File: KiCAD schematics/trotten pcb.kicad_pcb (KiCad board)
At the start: 2 copper layers, 151 x 114.3 mm, 19 parts, among them J1 Conn_HRCU4_main, J2 Conn_screen_BRD_main, J3 Conn_screen_BRD_Slave, J4 Conn_01x04_Socket, J5 Conn_02x03_Odd_Even, SW1 Haut, SW2 Bas, SW3 MEM_1, SW4 MEM_2, U1 std:8a282036eb974780bd16e9b19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, U2 BOB-12009, U3 ADAFRUIT-ESP32-S3, U7 INA260

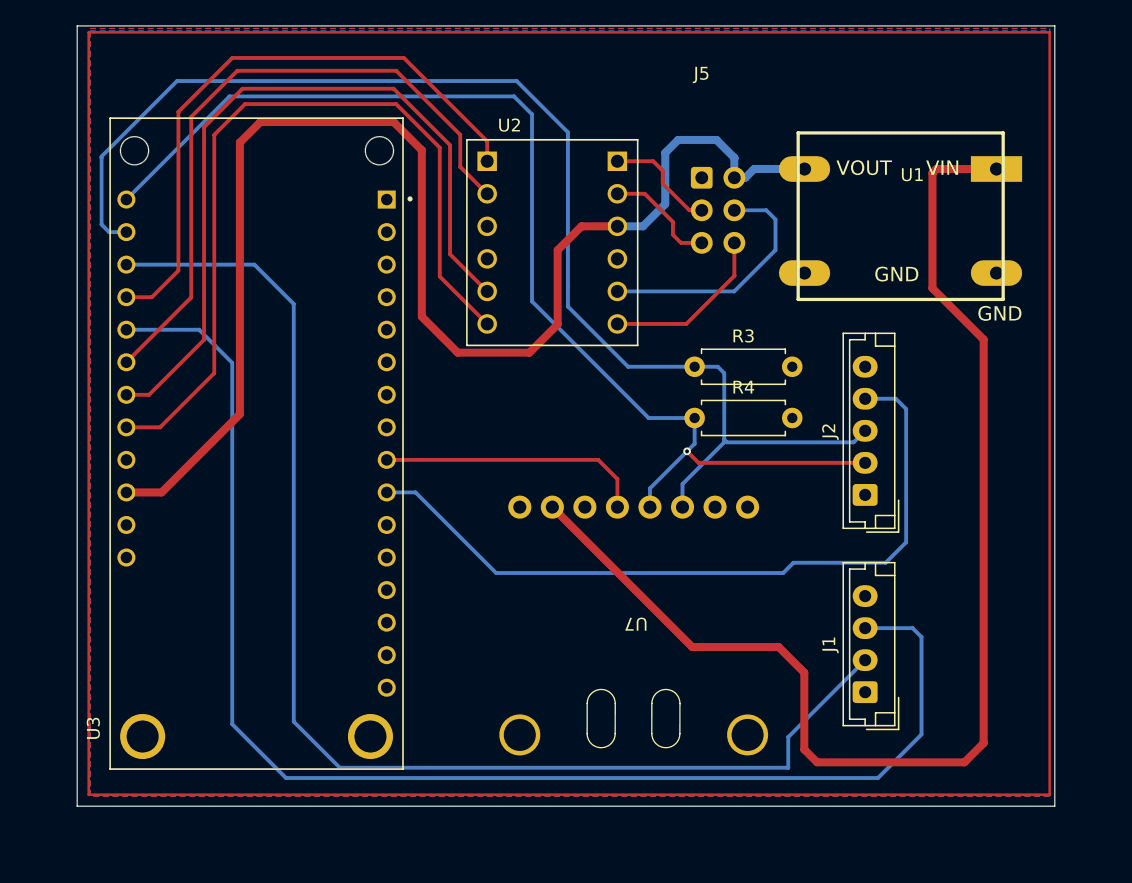
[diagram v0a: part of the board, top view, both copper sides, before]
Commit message: commencé le moteur
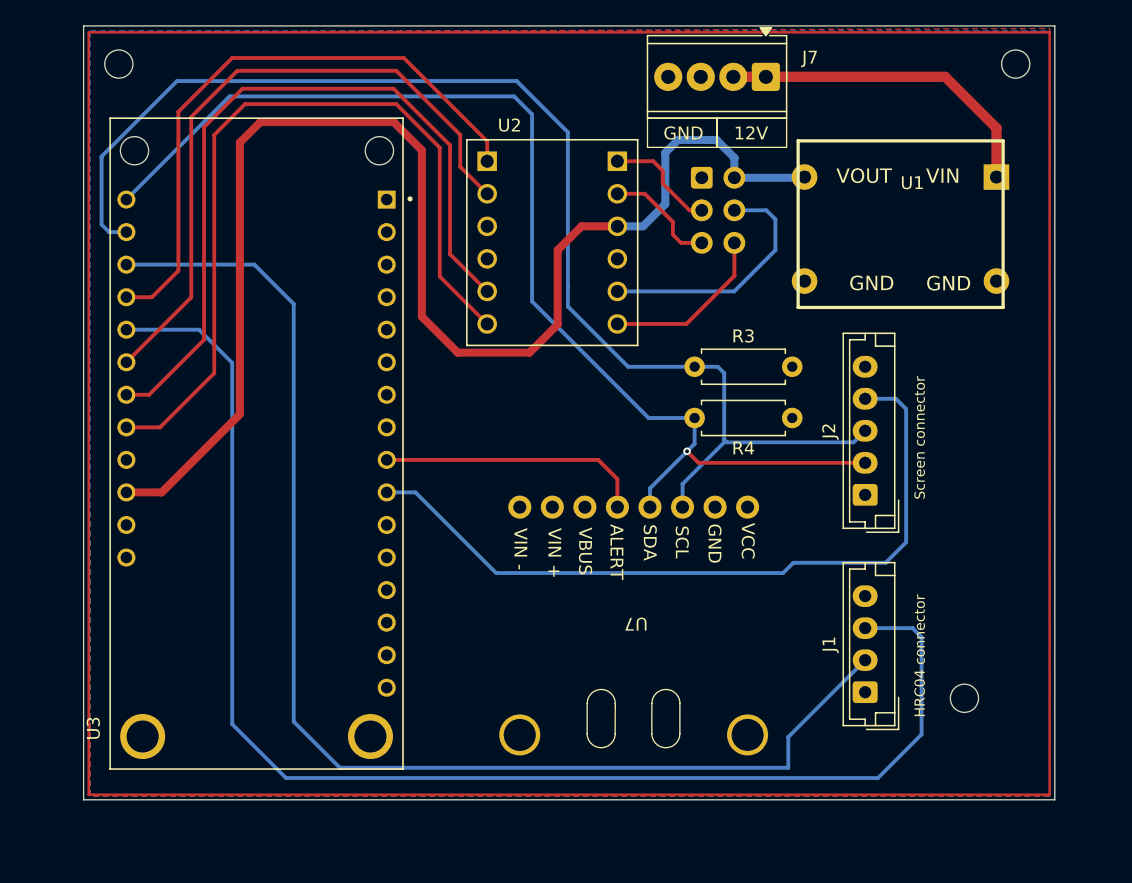
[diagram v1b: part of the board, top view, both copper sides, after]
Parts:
- added J7: Screw_Terminal_01x04, TerminalBlock_Phoenix:TerminalBlock_Phoenix_MPT-0,5-4-2.54_1x04_P2.54mm_Horizontal, F.Cu at (130.2, 27.9)
- added REF**: MountingHole_2.2mm_M2, MountingHole:MountingHole_2.2mm_M2, F.Cu at (79.8, 26.9)
- added REF**: MountingHole_2.2mm_M2, MountingHole:MountingHole_2.2mm_M2, F.Cu at (149.8, 26.9)
- added REF**: MountingHole_2.2mm_M2, MountingHole:MountingHole_2.2mm_M2, F.Cu at (145.8, 76.4)
- U1: value std:8a282036eb974780bd16e9b19a8357be -> S09-EY9-DC-DC
- moved U1 0.62 mm to (140.8, 39.4)
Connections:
- U7 pad 1: +12V -> unconnected-(U7-IN+-Pad1)
- U7 pad 10: (no net) -> +3.3V
- U7 pad 12: (no net) -> unconnected-(U7-VBUS-Pad12)
- U7 pad 14: (no net) -> Net-(U7-IN--Pad14)
- U7 pad 9: (no net) -> SCL - GP22
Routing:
- net +12V: track 97.3 -> 26.5 mm
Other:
- outline, holes or cut-outs redrawn
- board text added: "12V"
- board text added: "GND"
- board text added: "HRC04 connector"
- board text added: "Screen connector"
